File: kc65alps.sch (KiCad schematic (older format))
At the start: 160 parts, among them J1 Conn_01x04, J2 AVR-ISP-6, U1 ATmega32U4-AU, Y1 16MHz

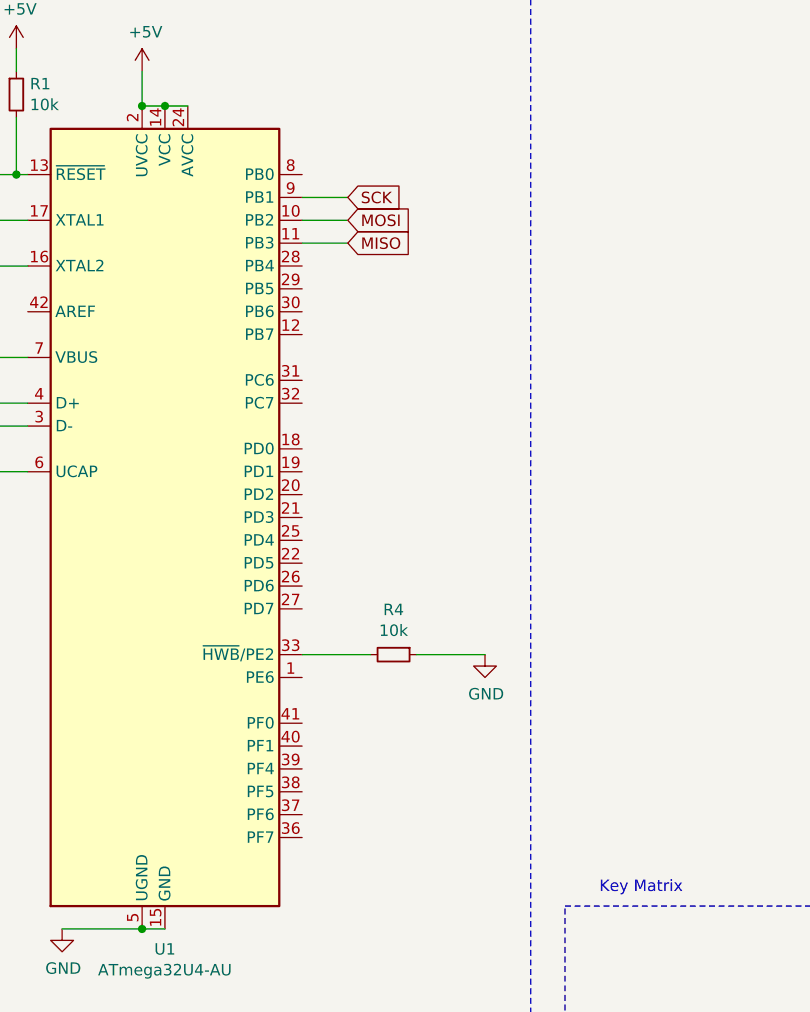
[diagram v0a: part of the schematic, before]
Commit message: PCB Update
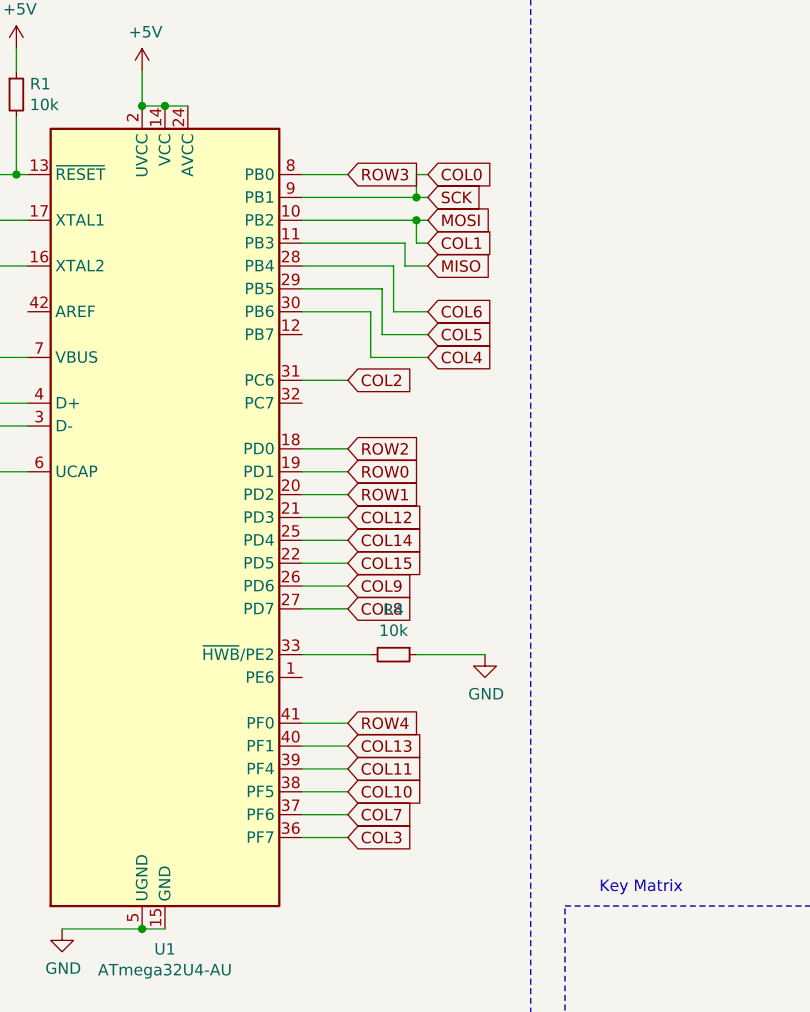
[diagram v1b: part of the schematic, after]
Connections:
- net MOSI is gone; now on net COL1: J2.4 (MOSI), U1.10 (PB2)
- net SCK is gone; now on net COL0: J2.3 (SCK), U1.9 (PB1)
- net COL10: now also U1.38 (PF5)
- net COL11: now also U1.39 (PF4)
- net COL12: now also U1.21 (PD3)
- net COL13: now also U1.40 (PF1)
- net COL14: now also U1.25 (PD4)
- net COL15: now also U1.22 (PD5)
- net COL2: now also U1.31 (PC6)
- net COL3: now also U1.36 (PF7)
- net COL4: now also U1.30 (PB6)
- net COL5: now also U1.29 (PB5)
- net COL6: now also U1.28 (PB4)
- net COL7: now also U1.37 (PF6)
- net COL8: now also U1.27 (PD7)
- net COL9: now also U1.26 (PD6)
- net ROW0: now also U1.19 (PD1)
- net ROW1: now also U1.20 (PD2)
- net ROW2: now also U1.18 (PD0)
- net ROW3: now also U1.8 (PB0)
- net ROW4: now also U1.41 (PF0)
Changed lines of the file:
@@
 $EndDescr
-$Comp
-L MCU_Microchip_ATmega:ATmega32U4-AU U1
-U 1 1 5DF6F14B
-P 2600 3100
-F 0 "U1" H 2600 1211 50  0000 C CNN
-F 1 "ATmega32U4-AU" H 2600 1120 50  0000 C CNN
-F 2 "Housings_QFP:TQFP-44_10x10mm_Pitch0.8mm" H 2600 3100 50  0001 C CIN
-F 3 "http://ww1.microchip.com/downloads/en/DeviceDoc/Atmel-7766-8-bit-AVR-ATmega16U4-32U4_Datasheet.pdf" H 2600 3100 50  0001 C CNN
-	1    2600 3100
-	1    0    0    -1
-$EndComp
 $Comp
 L power:+5V #PWR0101
@@
 Wire Wire Line
 	1700 1600 1950 1600
-Text GLabel 3400 1900 2    50   Input ~ 0
+Text GLabel 3750 2000 2    50   Input ~ 0
 MISO
-Text GLabel 3400 1800 2    50   Input ~ 0
+Text GLabel 3750 1800 2    50   Input ~ 0
 MOSI
-Text GLabel 3400 1700 2    50   Input ~ 0
+Text GLabel 3750 1700 2    50   Input ~ 0
 SCK
-Wire Wire Line
-	3200 1700 3400 1700
-Wire Wire Line
-	3400 1800 3200 1800
-Wire Wire Line
-	3200 1900 3400 1900
 $Comp
 L Connector:AVR-ISP-6 J2
@@
 	14600 5700 14600 5900
 Connection ~ 14600 5900
+Text GLabel 3400 1600 2    50   Input ~ 0
+ROW3
+Wire Wire Line
+	3200 1600 3400 1600
+Text GLabel 3750 1600 2    50   Input ~ 0
+COL0
+Text GLabel 3750 1900 2    50   Input ~ 0
+COL1
+Text GLabel 3400 2500 2    50   Input ~ 0
+COL2
+Wire Wire Line
+	3700 1600 3700 1700
+Wire Wire Line
+	3700 1700 3200 1700
+Wire Wire Line
+	3700 1600 3750 1600
+Wire Wire Line
+	3700 1700 3750 1700
+Connection ~ 3700 1700
+Wire Wire Line
+	3200 1800 3700 1800
+Wire Wire Line
+	3700 1800 3700 1900
+Wire Wire Line
+	3700 1900 3750 1900
+Connection ~ 3700 1800
+Wire Wire Line
+	3700 1800 3750 1800
+Wire Wire Line
+	3650 1900 3650 2000
+Wire Wire Line
+	3200 1900 3650 1900
+Text GLabel 3400 2900 2    50   Input ~ 0
+ROW0
+Text GLabel 3400 3000 2    50   Input ~ 0
+ROW1
+Text GLabel 3400 2800 2    50   Input ~ 0
+ROW2
+Wire Wire Line
+	3200 2800 3400 2800
+Wire Wire Line
+	3200 2900 3400 2900
+Wire Wire Line
+	3200 3000 3400 3000
+Text GLabel 3400 4000 2    50   Input ~ 0
+ROW4
+Wire Wire Line
+	3400 4000 3200 4000
+Text GLabel 3400 4400 2    50   Input ~ 0
+COL7
+Text GLabel 3400 4300 2    50   Input ~ 0
+COL10
+Text GLabel 3400 4200 2    50   Input ~ 0
+COL11
+Text GLabel 3400 4100 2    50   Input ~ 0
+COL13
+Text GLabel 3400 4500 2    50   Input ~ 0
+COL3
+Wire Wire Line
+	3200 4100 3400 4100
+Wire Wire Line
+	3200 4200 3400 4200
+Wire Wire Line
+	3200 4300 3400 4300
+Wire Wire Line
+	3200 4400 3400 4400
+Wire Wire Line
+	3200 4500 3400 4500
+Text GLabel 3750 2400 2    50   Input ~ 0
+COL4
+Text GLabel 3750 2300 2    50   Input ~ 0
+COL5
+Text GLabel 3750 2200 2    50   Input ~ 0
+COL6
+Text GLabel 3400 3500 2    50   Input ~ 0
+COL8
+Text GLabel 3400 3400 2    50   Input ~ 0
+COL9
+Text GLabel 3400 3100 2    50   Input ~ 0
+COL12
+Text GLabel 3400 3200 2    50   Input ~ 0
+COL14
+Text GLabel 3400 3300 2    50   Input ~ 0
+COL15
+Wire Wire Line
+	3200 2000 3600 2000
+Wire Wire Line
+	3600 2000 3600 2200
+Wire Wire Line
+	3600 2200 3750 2200
+Wire Wire Line
+	3200 2100 3550 2100
+Wire Wire Line
+	3550 2100 3550 2300
+Wire Wire Line
+	3550 2300 3750 2300
+Wire Wire Line
+	3200 2200 3500 2200
+Wire Wire Line
+	3500 2200 3500 2400
+Wire Wire Line
+	3500 2400 3750 2400
+Wire Wire Line
+	3200 3100 3400 3100
+Wire Wire Line
+	3400 3200 3200 3200
+Wire Wire Line
+	3200 3300 3400 3300
+Wire Wire Line
+	3400 3400 3200 3400
+Wire Wire Line
+	3200 3500 3400 3500
+$Comp
+L MCU_Microchip_ATmega:ATmega32U4-AU U1
+U 1 1 5DF6F14B
+P 2600 3100
+F 0 "U1" H 2600 1211 50  0000 C CNN
+F 1 "ATmega32U4-AU" H 2600 1120 50  0000 C CNN
+F 2 "Housings_QFP:TQFP-44_10x10mm_Pitch0.8mm" H 2600 3100 50  0001 C CIN
+F 3 "http://ww1.microchip.com/downloads/en/DeviceDoc/Atmel-7766-8-bit-AVR-ATmega16U4-32U4_Datasheet.pdf" H 2600 3100 50  0001 C CNN
+	1    2600 3100
+	1    0    0    -1
+$EndComp
+Wire Wire Line
+	3200 2500 3400 2500
+Wire Wire Line
+	3650 2000 3750 2000
 $EndSCHEMATC

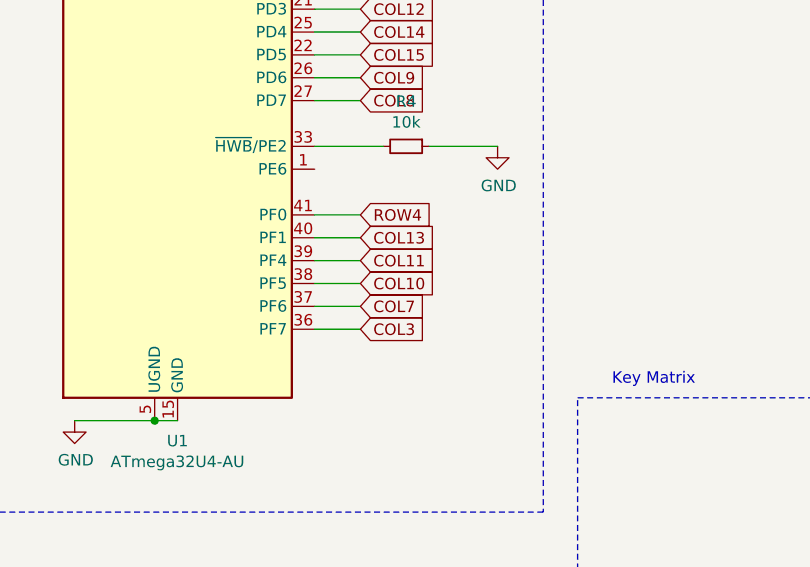
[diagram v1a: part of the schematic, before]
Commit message: PCB Update
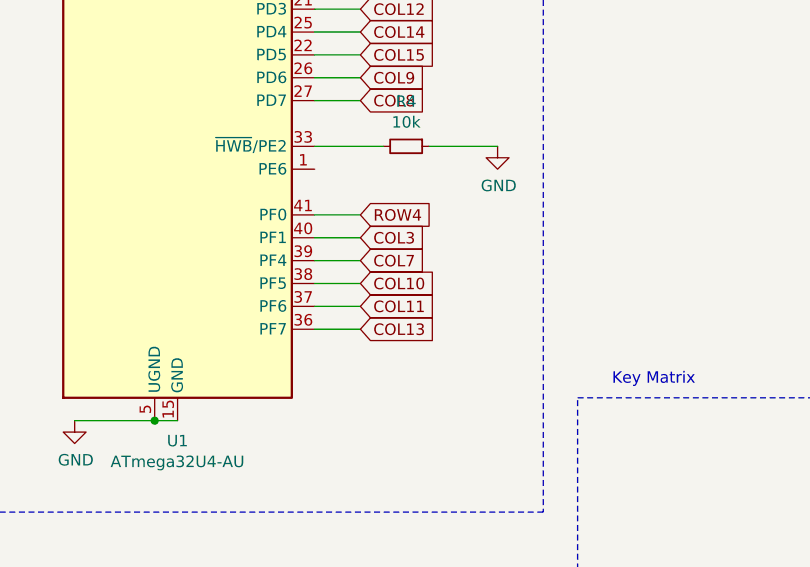
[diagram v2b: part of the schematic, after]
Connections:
- net COL11: now also U1.37 (PF6); no longer U1.39 (PF4)
- net COL13: now also U1.36 (PF7); no longer U1.40 (PF1)
- net COL3: now also U1.40 (PF1); no longer U1.36 (PF7)
- net COL7: now also U1.39 (PF4); no longer U1.37 (PF6)
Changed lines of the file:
@@
 Wire Wire Line
 	3400 4000 3200 4000
-Text GLabel 3400 4400 2    50   Input ~ 0
+Text GLabel 3400 4200 2    50   Input ~ 0
 COL7
 Text GLabel 3400 4300 2    50   Input ~ 0
 COL10
-Text GLabel 3400 4200 2    50   Input ~ 0
+Text GLabel 3400 4400 2    50   Input ~ 0
 COL11
+Text GLabel 3400 4500 2    50   Input ~ 0
+COL13
 Text GLabel 3400 4100 2    50   Input ~ 0
-COL13
-Text GLabel 3400 4500 2    50   Input ~ 0
 COL3
 Wire Wire Line
